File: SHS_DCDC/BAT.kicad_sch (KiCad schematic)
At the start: 11 parts, among them Q10 PMV100XPEAR, Q11 PMV100XPEAR, Q12 PMV100XPEAR, Q17 PMV100XPEAR, Q9 PMV100XPEAR, U2 INA181, U7 MCP101

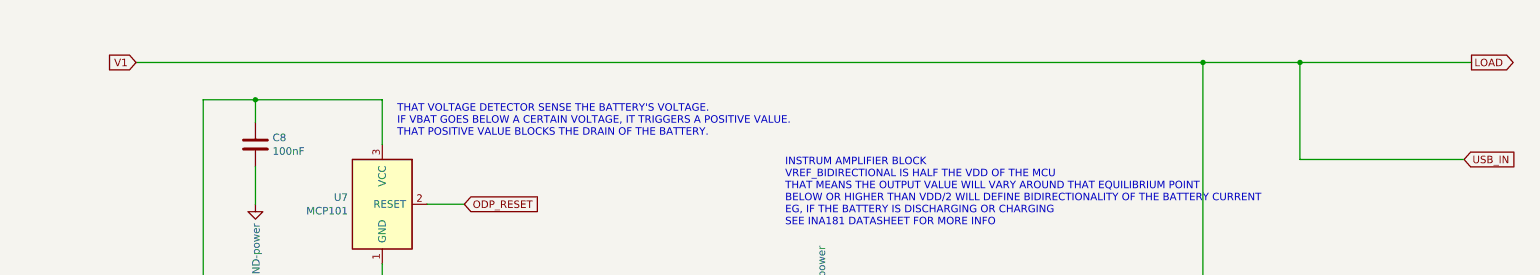
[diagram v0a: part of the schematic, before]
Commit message: Commit_190223
Normal commit
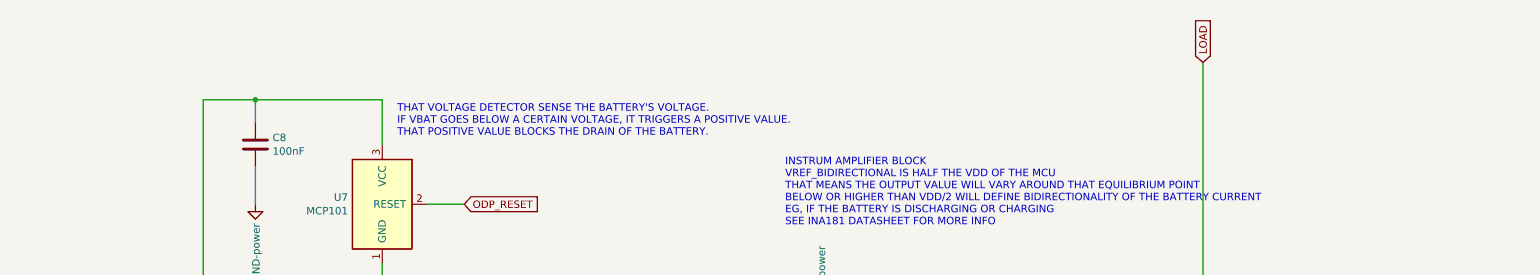
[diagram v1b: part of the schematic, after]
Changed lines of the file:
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@@
   (junction (at 217.17 76.2) (diameter 0) (color 0 0 0 0)
   )
-  (junction (at 233.68 30.48) (diameter 0) (color 0 0 0 0)
-  )
-  (junction (at 217.17 30.48) (diameter 0) (color 0 0 0 0)
-  )
   (junction (at 55.88 36.83) (diameter 0) (color 0 0 0 0)
   )
@@
     (stroke (width 0) (type default) (color 0 0 0 0))
   )
-  (wire (pts (xy 261.62 46.99) (xy 233.68 46.99))
-    (stroke (width 0) (type default) (color 0 0 0 0))
-  )
   (wire (pts (xy 217.17 76.2) (xy 217.17 83.82))
     (stroke (width 0) (type default) (color 0 0 0 0))
@@
     (stroke (width 0) (type default) (color 0 0 0 0))
   )
-  (wire (pts (xy 35.56 30.48) (xy 217.17 30.48))
-    (stroke (width 0) (type default) (color 0 0 0 0))
-  )
   (wire (pts (xy 55.88 48.26) (xy 55.88 54.61))
     (stroke (width 0) (type default) (color 0 0 0 0))
@@
     (stroke (width 0) (type default) (color 0 0 0 0))
   )
-  (wire (pts (xy 217.17 30.48) (xy 233.68 30.48))
-    (stroke (width 0) (type default) (color 0 0 0 0))
-  )
   (wire (pts (xy 95.25 171.45) (xy 95.25 181.61))
     (stroke (width 0) (type default) (color 0 0 0 0))
@@
     (stroke (width 0) (type default) (color 0 0 0 0))
   )
-  (wire (pts (xy 233.68 30.48) (xy 262.89 30.48))
-    (stroke (width 0) (type default) (color 0 0 0 0))
-  )
   (wire (pts (xy 115.57 151.13) (xy 95.25 151.13))
     (stroke (width 0) (type default) (color 0 0 0 0))
@@
   )
   (wire (pts (xy 46.99 151.13) (xy 64.77 151.13))
-    (stroke (width 0) (type default) (color 0 0 0 0))
-  )
-  (wire (pts (xy 233.68 46.99) (xy 233.68 30.48))
     (stroke (width 0) (type default) (color 0 0 0 0))
   )
@@
     (at 146.05 58.42 0)
     (effects (font (size 1.27 1.27)) (justify left bottom))
-  )
-  (global_label "USB_IN" (shape input) (at 261.62 46.99 0) (fields_autoplaced)
-    (effects (font (size 1.27 1.27)) (justify left))
-    (property "Intersheet References" "${INTERSHEET_REFS}" (id 0) (at 287.02 -176.53 0)
-      (effects (font (size 1.27 1.27)) hide)
-    )
   )
   (global_label "VREF_BIDIRECTIONAL" (shape input) (at 133.35 72.39 180) (fields_autoplaced)
@@
     )
   )
-  (global_label "LOAD" (shape output) (at 262.89 30.48 0) (fields_autoplaced)
-    (effects (font (size 1.27 1.27)) (justify left))
-    (property "Intersheet References" "${INTERSHEET_REFS}" (id 0) (at 0 -7.62 0)
-      (effects (font (size 1.27 1.27)) hide)
-    )
-  )
   (global_label "V_MCU" (shape input) (at 152.4 104.14 270) (fields_autoplaced)
     (effects (font (size 1.27 1.27)) (justify right))
@@
     )
   )
-  (global_label "V1" (shape input) (at 35.56 30.48 180) (fields_autoplaced)
-    (effects (font (size 1.27 1.27)) (justify right))
-    (property "Intersheet References" "${INTERSHEET_REFS}" (id 0) (at 30.9377 30.4006 0)
-      (effects (font (size 1.27 1.27)) (justify right) hide)
-    )
-  )
+  (global_label "LOAD" (shape input) (at 217.17 30.48 90) (fields_autoplaced)
+    (effects (font (size 1.27 1.27)) (justify left))
+    (property "Intersheet References" "${INTERSHEET_REFS}" (id 0) (at 217.2494 23.4387 90)
+      (effects (font (size 1.27 1.27)) (justify left) hide)
+    )
+  )
